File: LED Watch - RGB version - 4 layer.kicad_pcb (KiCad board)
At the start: 2 copper layers, 41.9 x 49.3 mm, 140 parts, among them J1 AVR-ISP-6, J2 Lipo, J3 Coin Cell, SW1 SW_DPST, SW2 SW_DPST, U10 B39D3RGB-F6C0001HOU1930, U100 B39D3RGB-F6C0001HOU1930, U101 B39D3RGB-F6C0001HOU1930, U102 B39D3RGB-F6C0001HOU1930, U103 B39D3RGB-F6C0001HOU1930, U104 B39D3RGB-F6C0001HOU1930, U105 B39D3RGB-F6C0001HOU1930, U106 B39D3RGB-F6C0001HOU1930, U107 B39D3RGB-F6C0001HOU1930, U108 B39D3RGB-F6C0001HOU1930, U109 B39D3RGB-F6C0001HOU1930, U11 B39D3RGB-F6C0001HOU1930, U110 B39D3RGB-F6C0001HOU1930, U111 B39D3RGB-F6C0001HOU1930, U112 B39D3RGB-F6C0001HOU1930, U113 B39D3RGB-F6C0001HOU1930, U114 B39D3RGB-F6C0001HOU1930, U115 B39D3RGB-F6C0001HOU1930, U116 B39D3RGB-F6C0001HOU1930, U117 B39D3RGB-F6C0001HOU1930, U118 B39D3RGB-F6C0001HOU1930, U119 B39D3RGB-F6C0001HOU1930, U12 B39D3RGB-F6C0001HOU1930, U120 B39D3RGB-F6C0001HOU1930, U121 B39D3RGB-F6C0001HOU1930, U122 B39D3RGB-F6C0001HOU1930, U123 B39D3RGB-F6C0001HOU1930, U124 B39D3RGB-F6C0001HOU1930, U125 B39D3RGB-F6C0001HOU1930, U126 B39D3RGB-F6C0001HOU1930, U127 B39D3RGB-F6C0001HOU1930, U128 B39D3RGB-F6C0001HOU1930, U129 B39D3RGB-F6C0001HOU1930, U13 B39D3RGB-F6C0001HOU1930, U130 B39D3RGB-F6C0001HOU1930, U131 B39D3RGB-F6C0001HOU1930, U132 B39D3RGB-F6C0001HOU1930, U133 B39D3RGB-F6C0001HOU1930, U134 BMI160, U135 ATmega165PA-M, U14 B39D3RGB-F6C0001HOU1930, U15 B39D3RGB-F6C0001HOU1930, U16 B39D3RGB-F6C0001HOU1930, U17 B39D3RGB-F6C0001HOU1930, U18 B39D3RGB-F6C0001HOU1930, U19 B39D3RGB-F6C0001HOU1930, U2 B39D3RGB-F6C0001HOU1930, U20 B39D3RGB-F6C0001HOU1930, U21 B39D3RGB-F6C0001HOU1930, U22 B39D3RGB-F6C0001HOU1930, U23 B39D3RGB-F6C0001HOU1930, U24 B39D3RGB-F6C0001HOU1930, U25 B39D3RGB-F6C0001HOU1930, U26 B39D3RGB-F6C0001HOU1930, U27 B39D3RGB-F6C0001HOU1930, U28 B39D3RGB-F6C0001HOU1930, U29 B39D3RGB-F6C0001HOU1930, U3 B39D3RGB-F6C0001HOU1930, U30 B39D3RGB-F6C0001HOU1930, U31 B39D3RGB-F6C0001HOU1930, U32 B39D3RGB-F6C0001HOU1930, U33 B39D3RGB-F6C0001HOU1930, U34 B39D3RGB-F6C0001HOU1930, U35 B39D3RGB-F6C0001HOU1930, U36 B39D3RGB-F6C0001HOU1930, U37 B39D3RGB-F6C0001HOU1930, U38 B39D3RGB-F6C0001HOU1930, U39 B39D3RGB-F6C0001HOU1930, U4 B39D3RGB-F6C0001HOU1930, U40 B39D3RGB-F6C0001HOU1930, U41 B39D3RGB-F6C0001HOU1930, U42 B39D3RGB-F6C0001HOU1930, U43 B39D3RGB-F6C0001HOU1930, U44 B39D3RGB-F6C0001HOU1930, U45 B39D3RGB-F6C0001HOU1930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

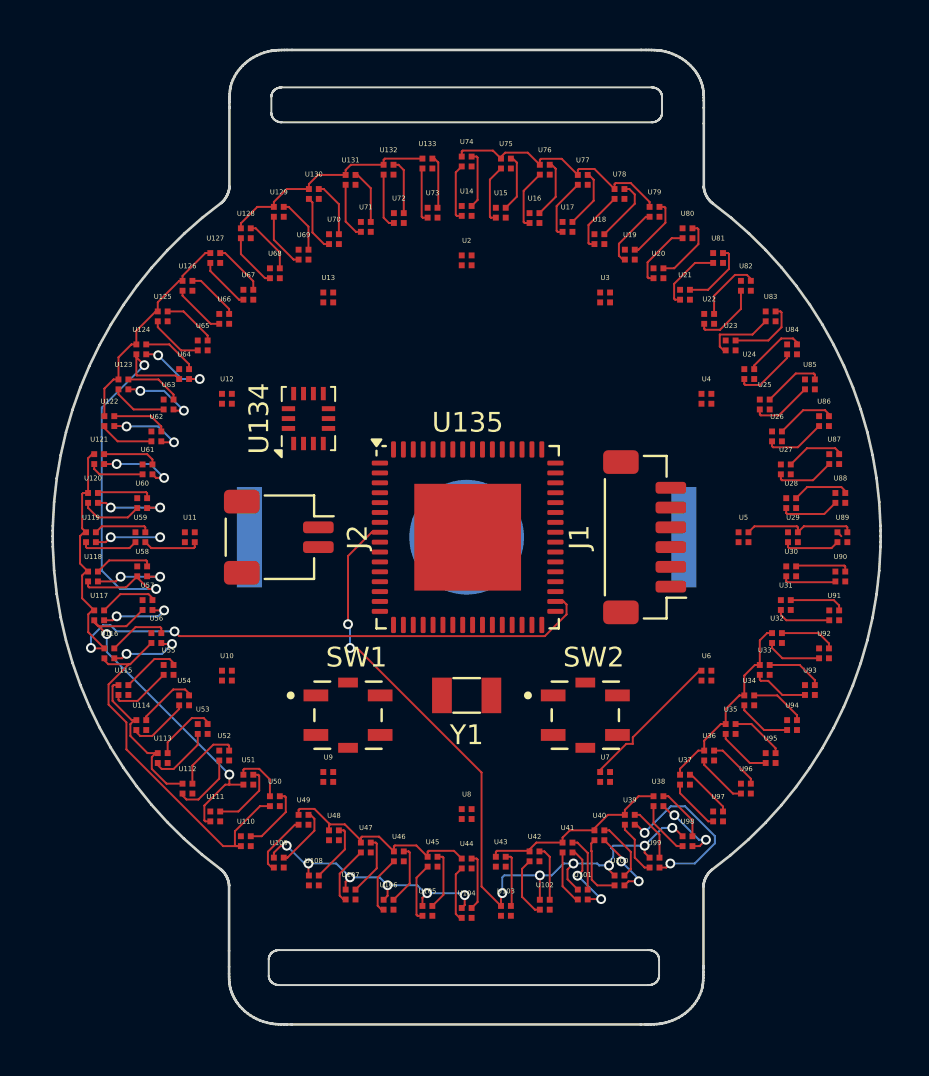
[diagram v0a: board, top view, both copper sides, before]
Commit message: added caps.. still unsuccessful routing
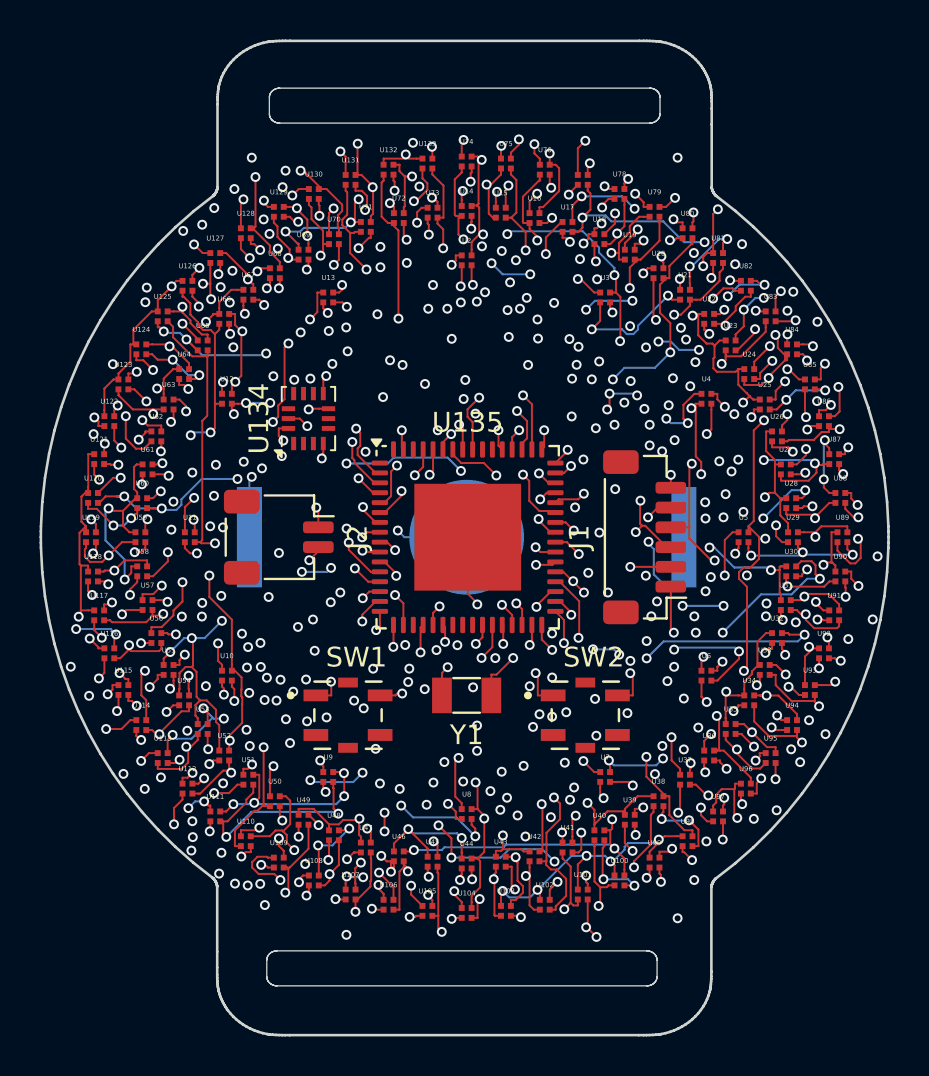
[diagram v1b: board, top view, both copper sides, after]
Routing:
- net /G5: track 3.91 -> 186.3 mm, vias 2 -> 38
- net /G6: track 3.99 -> 178.2 mm, vias 2 -> 39
- net /G4: track 10.2 -> 183.1 mm, vias 4 -> 33
- net /G2: track 16.7 -> 184.1 mm, vias 6 -> 28
- net /G3: track 11.3 -> 175.5 mm, vias 6 -> 34
- net /G1: track 11.5 -> 169.1 mm, vias 6 -> 29
- net /R6: track 28.8 -> 179.8 mm, vias 0 -> 40
- net /R1: track 29.8 -> 179.7 mm, vias 0 -> 31
- net /R3: track 30.4 -> 177.0 mm, vias 0 -> 28
- net /R4: track 32.9 -> 179.4 mm, vias 0 -> 39
- net /B5: track 26.6 -> 172.1 mm, vias 0 -> 32
- net /R2: track 30.2 -> 174.6 mm, vias 0 -> 34
- net /B6: track 26.2 -> 170.1 mm, vias 0 -> 33
- net /B4: track 29.9 -> 172.2 mm, vias 0 -> 27
- net /R5: track 29.1 -> 170.9 mm, vias 0 -> 33
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- added copper zone on In1.Cu, net Net-(J1-GND)
- added copper zone on In2.Cu, net Net-(J1-VCC)
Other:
- board size 41.9 x 49.3 mm -> 42.9 x 50.3 mm
- copper layers 2 -> 4
